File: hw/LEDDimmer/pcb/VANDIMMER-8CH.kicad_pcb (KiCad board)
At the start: 2 copper layers, 96.7 x 132.1 mm, 42 parts, among them J1 PWR_IN, J10 BTN1, J11 BTN2, J2 CH1, J3 CH2, J4 CH3, J5 CH4, J6 CH5, J7 CH6, J8 CH7, J9 CH8, Q1 IRLZ44N, Q2 IRLZ44N, Q3 IRLZ44N, Q4 IRLZ44N, Q5 IRLZ44N, Q6 IRLZ44N, Q7 IRLZ44N, Q8 IRLZ44N, U1 LM1117T-3.3, U2 ESP32-DevkitC-1

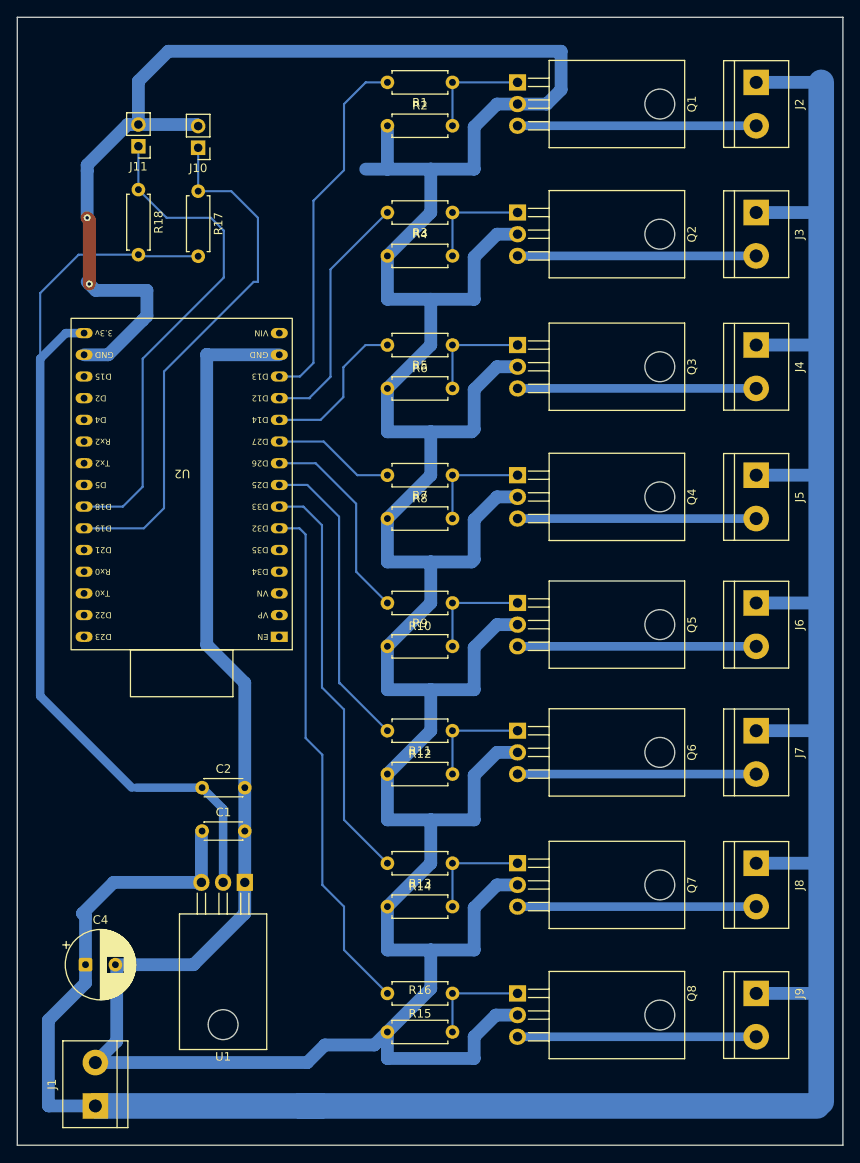
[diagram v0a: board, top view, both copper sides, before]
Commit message: hw
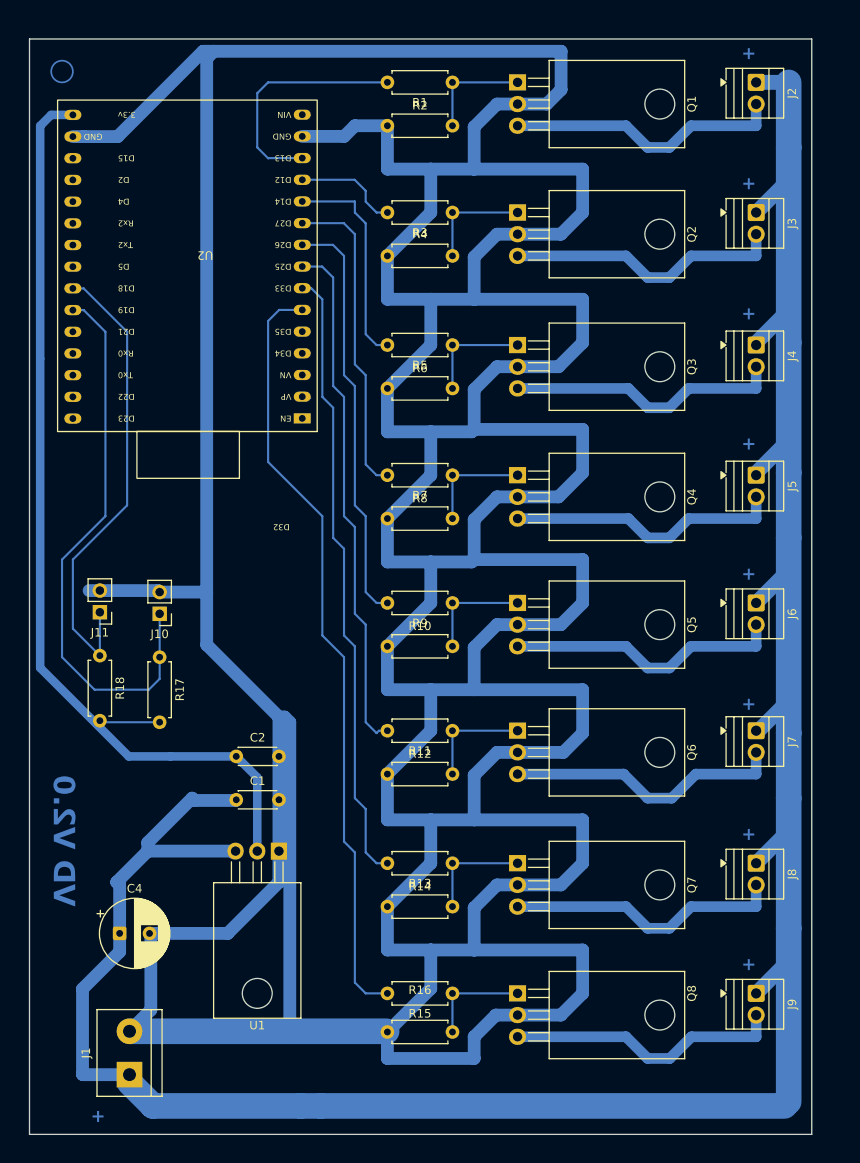
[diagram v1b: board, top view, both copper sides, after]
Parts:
- J2, J3, J4, J5, J6, J7, J8, J9: footprint TerminalBlock:TerminalBlock_bornier-2_P5.08mm -> TerminalBlock:TerminalBlock_Xinya_XY308-2.54-2P_1x02_P2.54mm_Horizontal
- moved J10 54.8 mm to (47.0, 102.9)
- moved J11 54.8 mm to (40.0, 102.7)
- moved R17 54.8 mm to (47.0, 108.0)
- moved R18 54.8 mm to (40.0, 107.8)
- moved U2 25.7 mm to (52.3, 60.4)
- moved C2 5.42 mm to (56.0, 119.6)
- moved C4 5.42 mm to (42.3, 140.3)
- moved J1 5.42 mm to (43.5, 156.8)
- moved U1 5.42 mm to (61.0, 130.7)
- moved C1 5.42 mm to (56.0, 124.7)
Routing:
- net GND: track 551.4 -> 772.6 mm, vias 2 -> 0
- net +3.3V: track 109.5 -> 140.9 mm
- net CH8: track 61.1 -> 90.5 mm
- net CH6: track 36.0 -> 61.0 mm
- net CH5: track 24.1 -> 48.9 mm
- net CH7: track 48.7 -> 72.8 mm
- net CH4: track 14.3 -> 37.2 mm
- net CH2: track 29.2 -> 12.3 mm
- net CH1: track 42.6 -> 27.9 mm
- net CH3: track 18.3 -> 25.3 mm
- net Net-(J7-Pin_2): track 27.9 -> 32.8 mm
- net Net-(J2-Pin_2): track 27.0 -> 31.7 mm
- net Net-(J6-Pin_2): track 27.9 -> 32.6 mm
- net Net-(J3-Pin_2): track 27.9 -> 32.6 mm
- net Net-(J9-Pin_2): track 27.9 -> 32.6 mm
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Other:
- board size 96.7 x 132.1 mm -> 91.6 x 128.3 mm
- board text added: "${REFERENCE}"
- board text added: "+"
- board text added: "D32"
- board text added: "VD V2.0"
